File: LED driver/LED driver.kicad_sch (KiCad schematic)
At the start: 45 parts, among them J1 Conn_VCC, J2 Conn_LED, J3 Conn_UART, J4 Conn_ESP32, P1 USB_C_Receptacle_USB2.0, Q1 IRFZ44NS, Q2 IRFZ44NS, Q3 IRFZ44NS, Q4 IRFZ44NS, Q5 IRFZ44NS, SW1 SW_Push, U1 ESP32-S2-WROVER-I, U2 MP2359

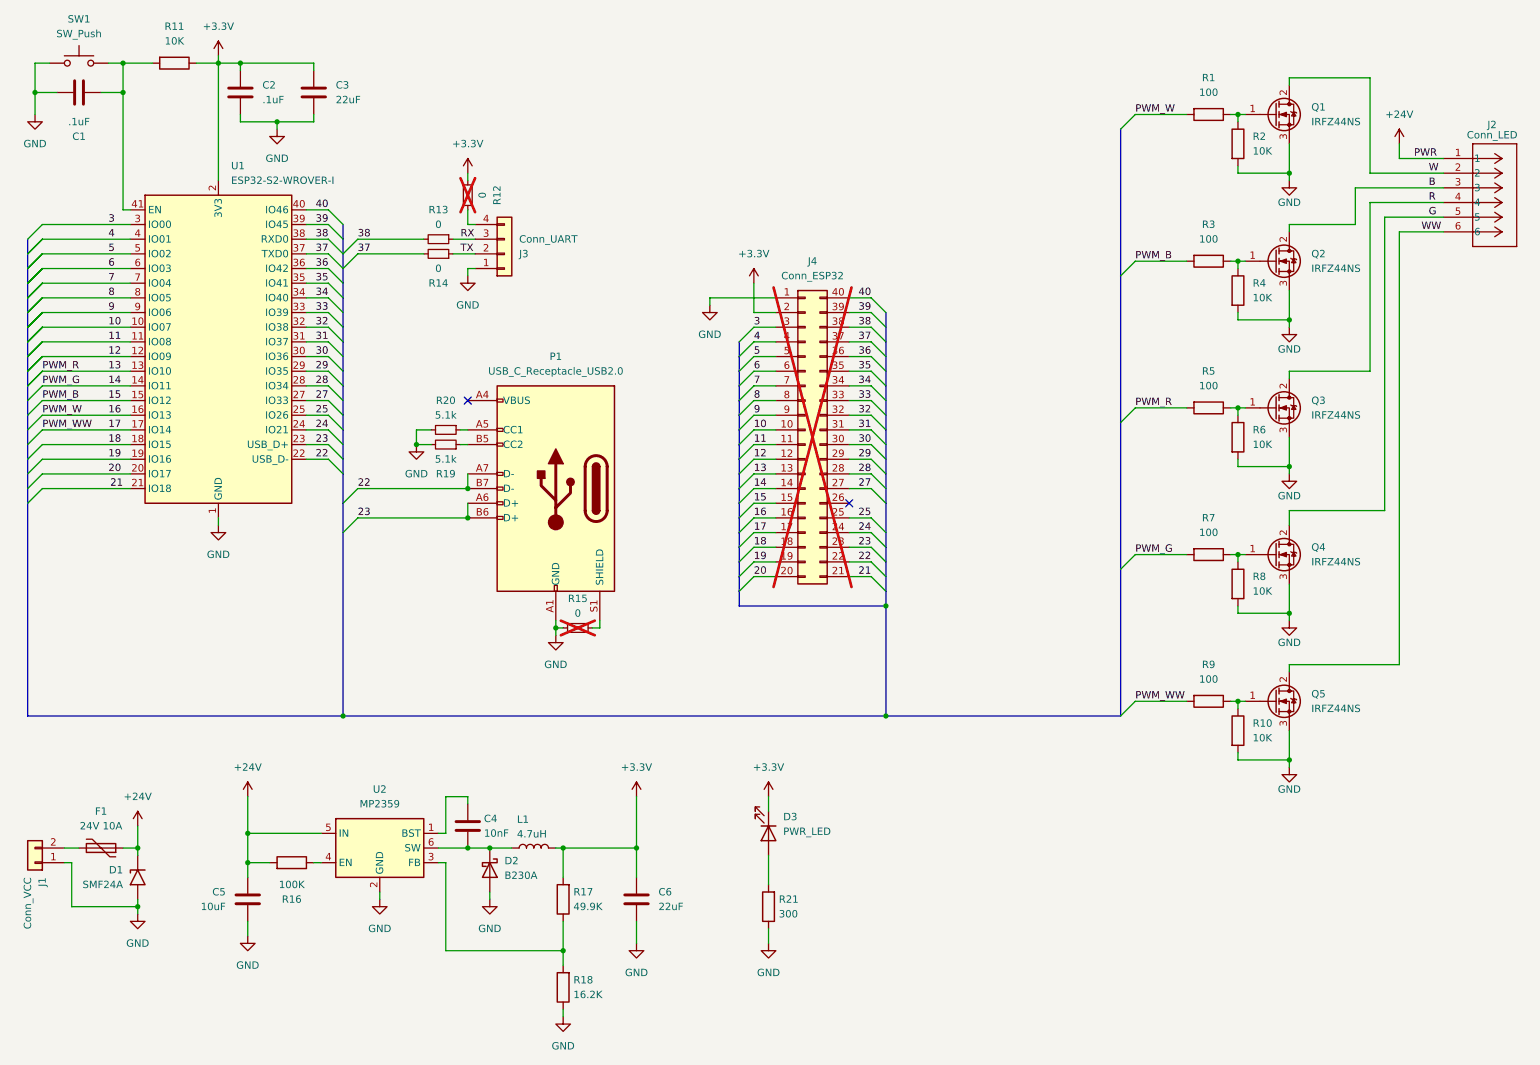
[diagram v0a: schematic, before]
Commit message: led driver
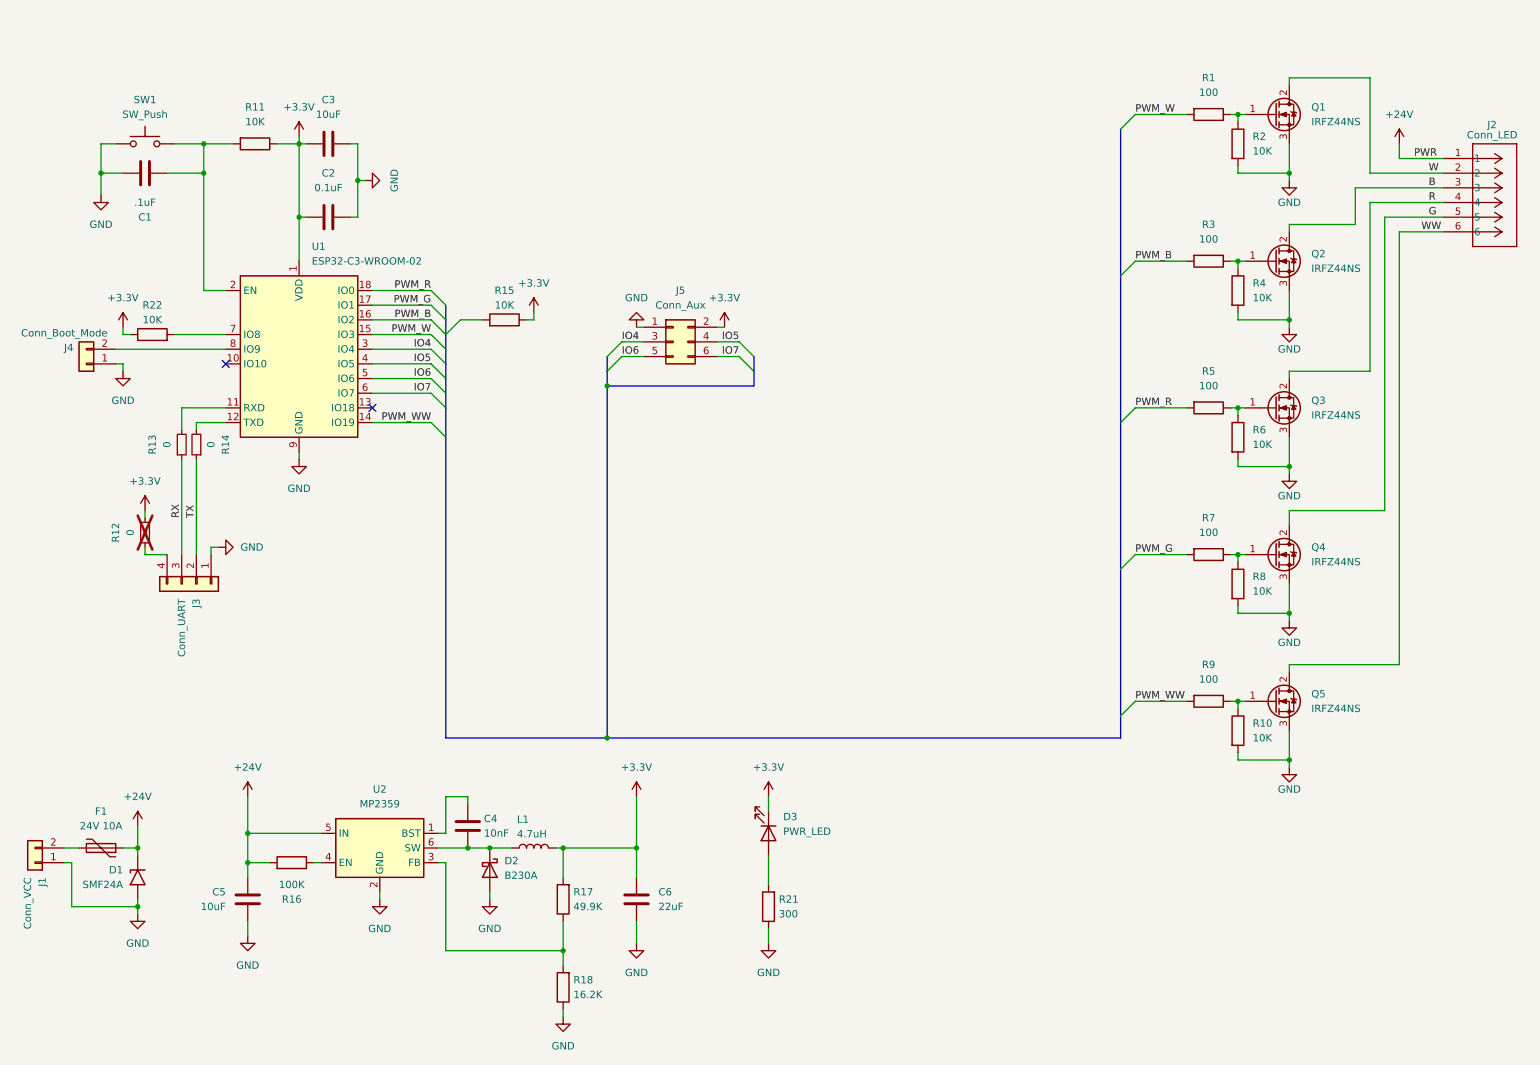
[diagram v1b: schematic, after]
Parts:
- removed J4: Conn_ESP32, Connector_PinSocket_2.54mm:PinSocket_2x20_P2.54mm_Vertical, symbol Connector_Generic:Conn_02x20_Counter_Clockwise
- removed P1: USB_C_Receptacle_USB2.0, Connector_USB:USB_C_Receptacle_GCT_USB4105-xx-A_16P_TopMnt_Horizontal, symbol Connector:USB_C_Receptacle_USB2.0_14P
- removed R15: 0, Resistor_SMD:R_0603_1608Metric_Pad0.98x0.95mm_HandSolder, symbol Device:R_Small
- removed R19, R20: 5.1k, Custom:R_0603_HandSolder_ValuePrinted, symbol Device:R_Small
- added J4: Conn_Boot_Mode, Connector_PinHeader_2.54mm:PinHeader_1x02_P2.54mm_Vertical, symbol Connector_Generic:Conn_01x02
- added J5: Conn_Aux, Connector_PinSocket_2.54mm:PinSocket_2x03_P2.54mm_Vertical, symbol Connector_Generic:Conn_02x03_Odd_Even
- added R15, R22: 10K, Custom:R_0603_HandSolder_ValuePrinted, symbol Device:R
- C2: value .1uF -> 0.1uF
- C3: value 22uF -> 10uF
- J2: footprint CON_532540670_MOL -> footprints:CON_532540670_MOL
- U1: value ESP32-S2-WROVER-I -> ESP32-C3-WROOM-02; footprint Custom:ESP32-S2-WROVER -> RF_Module:ESP32-C3-WROOM-02; symbol RF_Module:ESP32-S2-WROVER-I -> Custom:ESP32-C3-WROOM-02
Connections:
- net 19 is gone; now on net GND: U1.19 (GND)
- net 9 is gone; now on net GND: U1.9 (GND)
- net +3.3V: now also C2.2, C3.2, U1.1 (VDD), J5.2 (Pin_2), R15.1, R22.1; no longer C2.1, C3.1, U1.2 (3V3)
- net GND: now also C2.1, C3.1, J4.1 (Pin_1), J5.1 (Pin_1); no longer C2.2, C3.2, U1.1 (GND), U1.26 (GND), U1.42 (GND), U1.43 (GND)
- net at C1.2, R11.2, SW1.2: now also U1.2 (EN); no longer U1.41 (EN)
- net 10: no longer names the net of U1.10 (IO10)
- net 11: no longer names the net of U1.11 (RXD)
- net 11: now also R13.2
- net 12: no longer names the net of U1.12 (TXD)
- net 12: now also R14.2
- net 13: no longer names the net of U1.13 (IO18)
- net 13: no longer R5.2
- net 14 renamed PWM_G
- net PWM_G: now also U1.17 (IO1); no longer U1.14 (IO11)
- net 15 renamed PWM_B
- net PWM_B: now also U1.16 (IO2); no longer U1.15 (IO12)
- net 16 renamed PWM_W
- net PWM_W: now also U1.15 (IO3); no longer U1.16 (IO13)
- net 17 renamed PWM_WW
- net PWM_WW: now also U1.14 (IO19); no longer U1.17 (IO14)
- net 18 renamed PWM_R
- net PWM_R: now also R5.2
- removed net 20: U1.20 (IO17)
- removed net 21: U1.21 (IO18)
- removed net 22: U1.22 (USB_D-)
- removed net 23: U1.23 (USB_D+)
- removed net 24: U1.24 (IO21)
- removed net 25: U1.25 (IO26)
- removed net 27: U1.27 (IO33)
- removed net 28: U1.28 (IO34)
- removed net 29: U1.29 (IO35)
- net 3 renamed IO4
- net IO4: now also J5.3 (Pin_3)
- removed net 30: U1.30 (IO36)
- removed net 31: U1.31 (IO37)
- removed net 32: U1.32 (IO38)
- removed net 33: U1.33 (IO39)
- removed net 34: U1.34 (IO40)
- removed net 35: U1.35 (IO41)
- removed net 36: U1.36 (IO42)
- removed net 37: R14.2, U1.37 (TXD0)
- removed net 38: R13.2, U1.38 (RXD0)
- removed net 39: U1.39 (IO45)
- net 4 renamed IO5
- net IO5: now also J5.4 (Pin_4)
- removed net 40: U1.40 (IO46)
- net 5 renamed IO6
- net IO6: now also J5.5 (Pin_5)
- net 6 renamed IO7
- net IO7: now also J5.6 (Pin_6)
- net 7: no longer names the net of U1.7 (IO8)
- net 7: now also R22.2
- net 8: no longer names the net of U1.8 (IO9)
- net 8: now also J4.2 (Pin_2)
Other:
- moved on the sheet: C1, C3, J3, R11, R12, R13, R14, SW1
